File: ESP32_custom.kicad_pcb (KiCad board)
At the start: 4 copper layers, 32 x 50.3 mm, 26 parts, among them J1 TYPE-C-31-M-12, J2 Conn_01x16_Pin, J3 Conn_01x16_Pin, Q1 SS8050, Q2 SS8050, SW1 SW_Push, SW2 SW_Push, U2 ESP32-WROOM-32E 8MB, U3 CH340C, U4 AMS1117-3.3

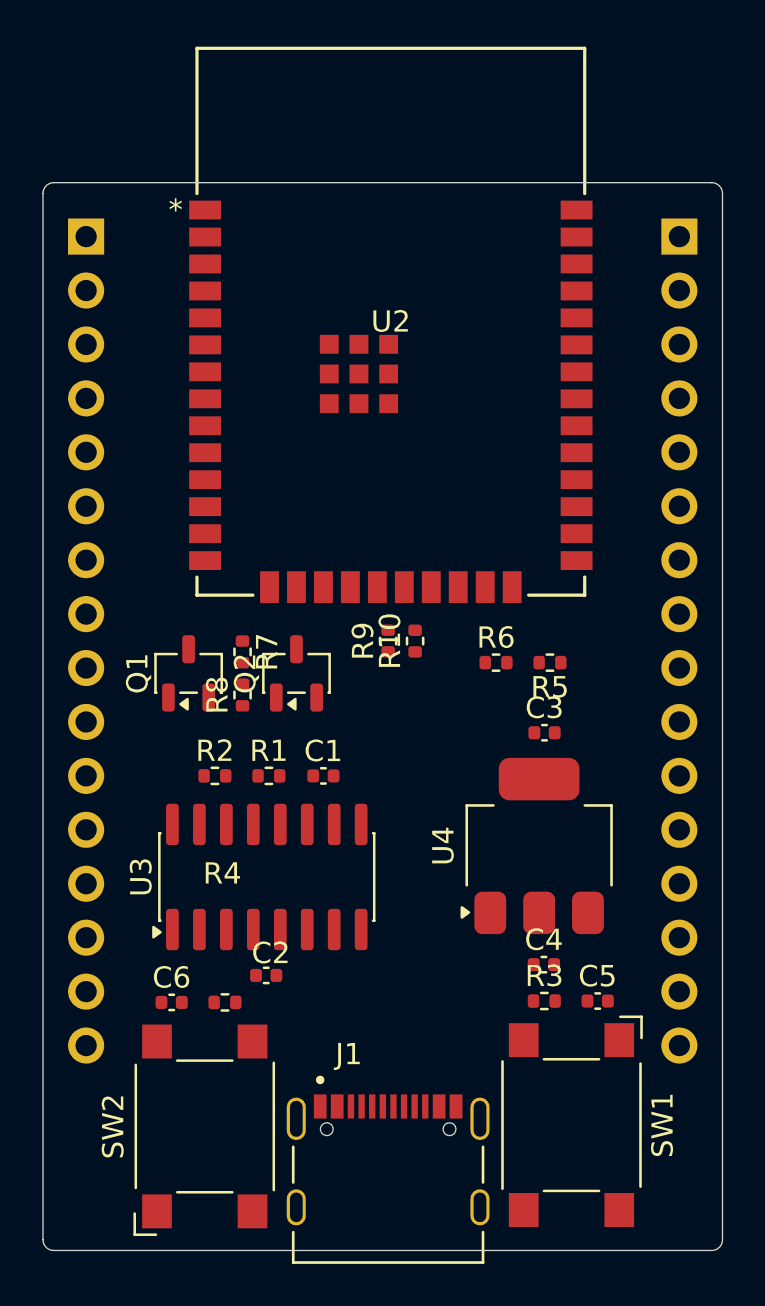
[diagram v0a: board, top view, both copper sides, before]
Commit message: Put trace and Put net classes (uncomplete)
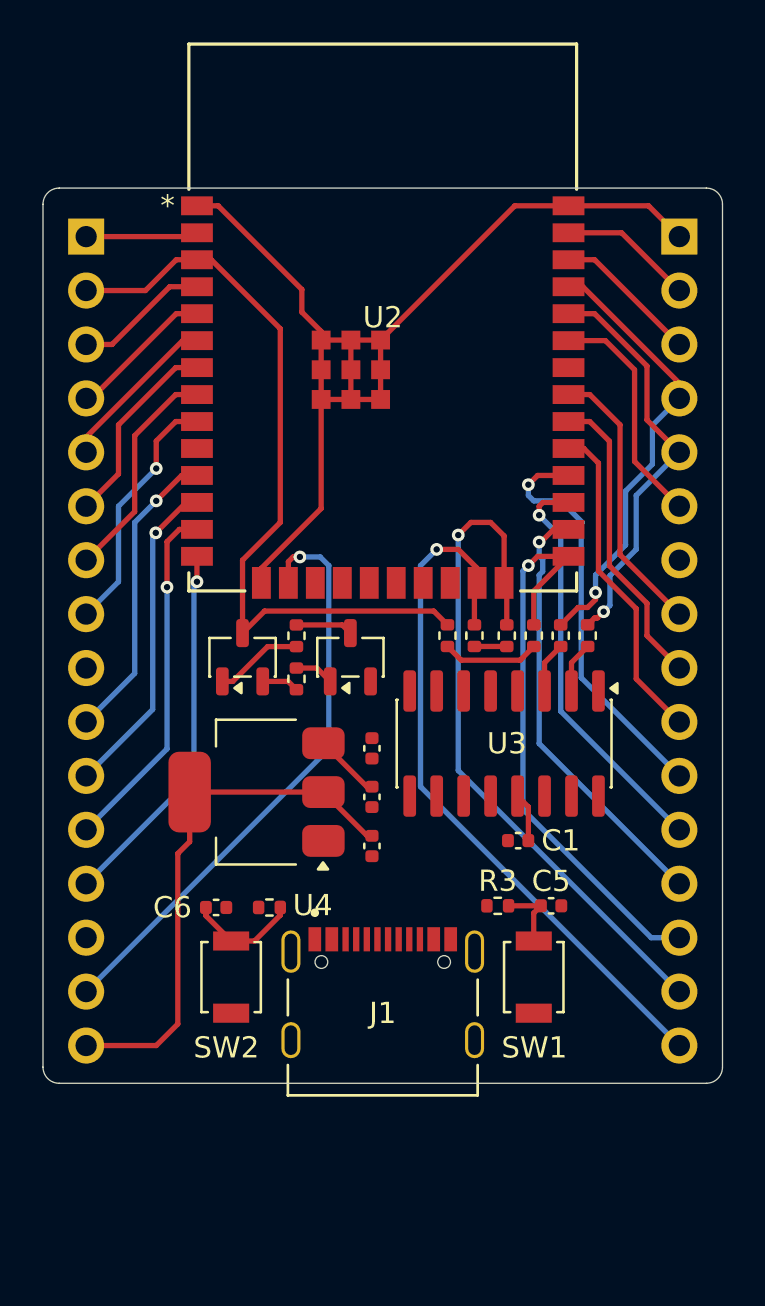
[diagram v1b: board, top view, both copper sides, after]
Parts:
- SW1, SW2: footprint Button_Switch_SMD:SW_SPST_Omron_B3FS-100xP -> Button_Switch_SMD:SW_SPST_B3U-1000P
- moved R2 18.8 mm to (137.9, 81.8), turned to 90 degrees
- moved R1 15.2 mm to (136.7, 81.8), turned to 90 degrees
- moved U4 13.6 mm to (122.3, 89.2), turned to 180 degrees
- moved U3 12.8 mm to (134.0, 86.9), turned to -90 degrees
- moved C2 11.8 mm to (127.8, 87.1), turned to -90 degrees
- moved C4 11.3 mm to (127.8, 89.4), turned to 90 degrees
- moved C3 9.72 mm to (127.8, 91.7), turned to -90 degrees
- moved C1 9.67 mm to (134.6, 91.4), turned to 180 degrees
- moved J1 7.88 mm to (128.3, 100.8)
- moved SW1 7.19 mm to (135.4, 97.9)
- moved SW2 7.14 mm to (121.1, 97.9), turned to -90 degrees
- moved C5 4.99 mm to (136.2, 94.5)
- moved R3 4.99 mm to (133.7, 94.5)
- moved C6 4.94 mm to (120.4, 94.6)
- moved R4 4.94 mm to (122.9, 94.6)
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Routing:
- net GND: track 0.00 -> 51.9 mm
- net /EN: track 0.00 -> 36.5 mm
- net +5V: track 0.00 -> 35.2 mm
- net /IO15: track 0.00 -> 33.7 mm, vias 0 -> 1
- net /IO2: track 0.00 -> 32.7 mm, vias 0 -> 1
- net /IO13: track 0.00 -> 28.0 mm, vias 0 -> 1
- net /IO0: track 0.00 -> 27.4 mm, vias 0 -> 1
- net /RX: track 0.00 -> 21.1 mm, vias 0 -> 1
- net /IO4: track 0.00 -> 20.6 mm, vias 0 -> 1
- net /IO17: track 0.00 -> 19.5 mm, vias 0 -> 1
- net /IO16: track 0.00 -> 19.4 mm, vias 0 -> 1
- net /TX: track 0.00 -> 19.4 mm, vias 0 -> 1
- net /IO12: track 0.00 -> 17.6 mm, vias 0 -> 1
- net /IO14: track 0.00 -> 16.8 mm, vias 0 -> 1
- net /IO5: track 0.00 -> 15.5 mm
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- added copper zone on In1.Cu, net GND
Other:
- board size 32 x 50.3 mm -> 32 x 42.2 mm
